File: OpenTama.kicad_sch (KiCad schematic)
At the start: 62 parts, among them J1 Conn_01x09, J2 Conn_01x14, J3 Conn_01x07, J4 USB_C_Receptacle_USB2.0, J5 Conn_01x14, Q1 BSS138, Q2 BSS138, Q3 BSS84, SW1 LEFT, SW2 MIDDLE, SW3 RIGHT, U1 TPS62203DBV, U2 LTC4054ES5-4.2, U3 STM32L072CBTx, U4 USBLC6-2SC6, Y1 32768Hz - 12,5 pF

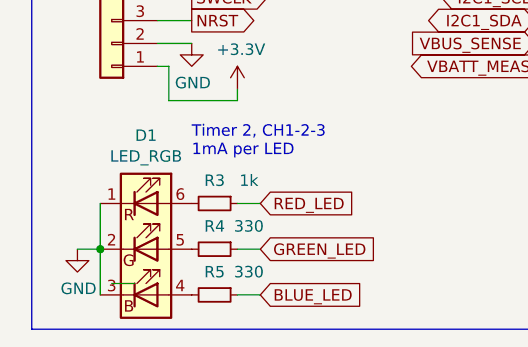
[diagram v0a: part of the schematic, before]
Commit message: Fix project (ERC)
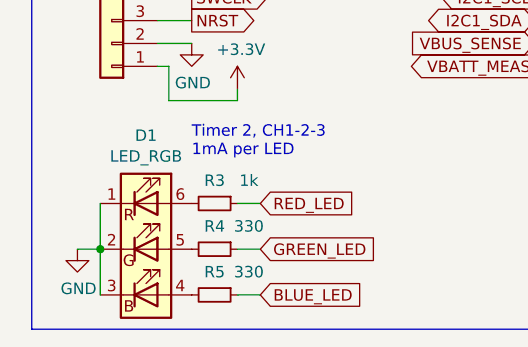
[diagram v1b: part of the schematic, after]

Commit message: Add JLCRotOffset (thx kabili207)
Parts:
- D1, J2, LS1, Q1, Q2, Q3, U1: JLCRotOffset (none) -> 180
- U2, U3, U4: JLCRotOffset (none) -> -90
